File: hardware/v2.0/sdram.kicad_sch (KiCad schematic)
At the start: 10 parts, among them IC1 IS42S16160J-6BLI, U1 ECP5-CABGA256

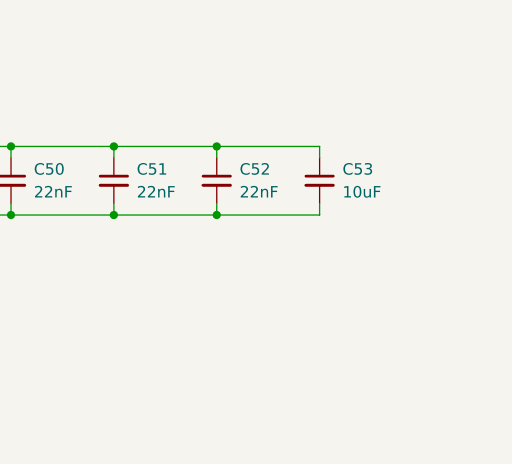
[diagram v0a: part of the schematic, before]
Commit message: Power lines
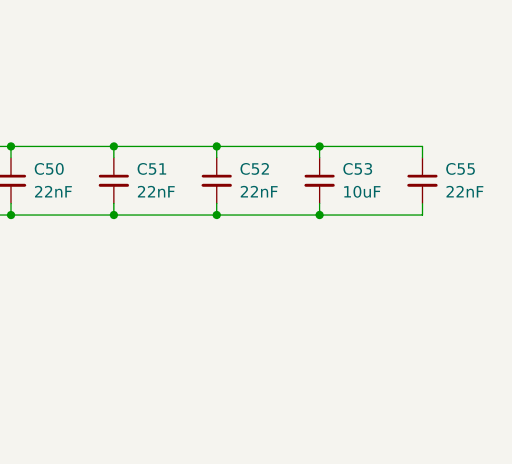
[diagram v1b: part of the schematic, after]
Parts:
- added C55: 22nF, Capacitor_SMD:C_0603_1608Metric, symbol Device:C_Small
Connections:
- net +3V3: now also C55.1
- net GND: now also C55.2
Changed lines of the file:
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@@
 	)
 	(junction
+		(at 264.16 39.37)
+		(diameter 0)
+		(color 0 0 0 0)
+	)
+	(junction
 		(at 53.34 58.42)
 		(diameter 0)
@@
 	)
 	(junction
+		(at 264.16 46.99)
+		(diameter 0)
+		(color 0 0 0 0)
+	)
+	(junction
 		(at 218.44 39.37)
 		(diameter 0)
@@
 	(wire
 		(pts
+			(xy 264.16 39.37) (xy 275.59 39.37)
+		)
+		(stroke
+			(width 0)
+			(type default)
+		)
+	)
+	(wire
+		(pts
 			(xy 54.61 125.73) (xy 60.96 125.73)
 		)
@@
 	(wire
 		(pts
+			(xy 275.59 46.99) (xy 275.59 45.72)
+		)
+		(stroke
+			(width 0)
+			(type default)
+		)
+	)
+	(wire
+		(pts
 			(xy 194.31 39.37) (xy 194.31 40.64)
 		)
@@
 	(wire
 		(pts
+			(xy 275.59 39.37) (xy 275.59 40.64)
+		)
+		(stroke
+			(width 0)
+			(type default)
+		)
+	)
+	(wire
+		(pts
 			(xy 157.48 100.33) (xy 162.56 100.33)
 		)
@@
 		)
 	)
+	(wire
+		(pts
+			(xy 264.16 46.99) (xy 275.59 46.99)
+		)
+		(stroke
+			(width 0)
+			(type default)
+		)
+	)
 	(bus
 		(pts
@@
 				)
 			)
+		)
+	)
+	(symbol
+		(lib_id "Device:C_Small")
+		(at 275.59 43.18 0)
+		(mirror y)
+		(unit 1)
+		(exclude_from_sim no)
+		(in_bom yes)
+		(on_board yes)
+		(dnp no)
+		(fields_autoplaced yes)
+		(property "Reference" "C55"
+			(at 278.13 41.9162 0)
+			(effects
+				(font
+					(size 1.27 1.27)
+				)
+				(justify right)
+			)
+		)
+		(property "Value" "22nF"
+			(at 278.13 44.4562 0)
+			(effects
+				(font
+					(size 1.27 1.27)
+				)
+				(justify right)
+			)
+		)
+		(property "Footprint" "Capacitor_SMD:C_0603_1608Metric"
+			(at 275.59 43.18 0)
+			(effects
+				(font
+					(size 1.27 1.27)
+				)
+				(hide yes)
+			)
+		)
+		(property "Datasheet" "~"
+			(at 275.59 43.18 0)
+			(effects
+				(font
+					(size 1.27 1.27)
+				)
+				(hide yes)
+			)
+		)
+		(property "Description" "Unpolarized capacitor, small symbol"
+			(at 275.59 43.18 0)
+			(effects
+				(font
+					(size 1.27 1.27)
+				)
+				(hide yes)
+			)
+		)
+		(property "LCSC Part #" "C77571"
+			(at 275.59 43.18 0)
+			(effects
+				(font
+					(size 1.27 1.27)
+				)
+				(hide yes)
+			)
+		)
+		(property "LCSC Link" "https://lcsc.com/product-detail/Multilayer-Ceramic-Capacitors-MLCC-SMD-SMT_Samsung-Electro-Mechanics-CL05B104KB54PNC_C307331.html"
+			(at 275.59 43.18 0)
+			(effects
+				(font
+					(size 1.27 1.27)
+				)
+				(hide yes)
+			)
+		)
+		(property "Manufactuer Part Number" "0603B223K500NT"
+			(at 275.59 43.18 0)
+			(effects
+				(font
+					(size 1.27 1.27)
+				)
+				(hide yes)
+			)
+		)
+		(property "Note" ""
+			(at 275.59 43.18 0)
+			(effects
+				(font
+					(size 1.27 1.27)
+				)
+				(hide yes)
+			)
+		)
+		(property "Notes" ""
+			(at 275.59 43.18 0)
+			(effects
+				(font
+					(size 1.27 1.27)
+				)
+				(hide yes)
+			)
+		)
+		(pin "1"
+		)
+		(pin "2"
+		)
+		(instances
+			(project "icepi-zero"
+				(path "/f88da08e-cf42-4d03-a08f-3f602fe6658d/3bffbb9a-e009-498c-a1b0-c490cdf30139"
+					(reference "C55")
+					(unit 1)
+				)
+			)

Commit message: Power lines done
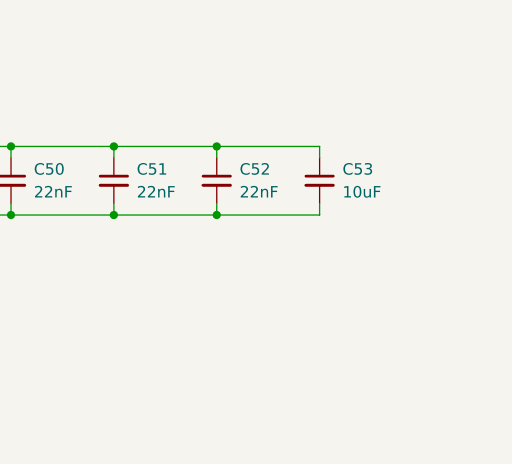
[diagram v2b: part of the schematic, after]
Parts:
- removed C55: 22nF, Capacitor_SMD:C_0603_1608Metric, symbol Device:C_Small
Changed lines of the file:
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@@
 	)
 	(junction
-		(at 264.16 39.37)
-		(diameter 0)
-		(color 0 0 0 0)
-	)
-	(junction
 		(at 53.34 58.42)
 		(diameter 0)
@@
 	)
 	(junction
-		(at 264.16 46.99)
-		(diameter 0)
-		(color 0 0 0 0)
-	)
-	(junction
 		(at 218.44 39.37)
 		(diameter 0)
@@
 	(wire
 		(pts
-			(xy 264.16 39.37) (xy 275.59 39.37)
-		)
-		(stroke
-			(width 0)
-			(type default)
-		)
-	)
-	(wire
-		(pts
 			(xy 54.61 125.73) (xy 60.96 125.73)
 		)
@@
 	(wire
 		(pts
-			(xy 275.59 46.99) (xy 275.59 45.72)
-		)
-		(stroke
-			(width 0)
-			(type default)
-		)
-	)
-	(wire
-		(pts
 			(xy 194.31 39.37) (xy 194.31 40.64)
 		)
@@
 	(wire
 		(pts
-			(xy 275.59 39.37) (xy 275.59 40.64)
-		)
-		(stroke
-			(width 0)
-			(type default)
-		)
-	)
-	(wire
-		(pts
 			(xy 157.48 100.33) (xy 162.56 100.33)
 		)
@@
 		)
 	)
-	(wire
-		(pts
-			(xy 264.16 46.99) (xy 275.59 46.99)
-		)
-		(stroke
-			(width 0)
-			(type default)
-		)
-	)
 	(bus
 		(pts
@@
 				)
 			)
-		)
-	)
-	(symbol
-		(lib_id "Device:C_Small")
-		(at 275.59 43.18 0)
-		(mirror y)
-		(unit 1)
-		(exclude_from_sim no)
-		(in_bom yes)
-		(on_board yes)
-		(dnp no)
-		(fields_autoplaced yes)
-		(property "Reference" "C55"
-			(at 278.13 41.9162 0)
-			(effects
-				(font
-					(size 1.27 1.27)
-				)
-				(justify right)
-			)
-		)
-		(property "Value" "22nF"
-			(at 278.13 44.4562 0)
-			(effects
-				(font
-					(size 1.27 1.27)
-				)
-				(justify right)
-			)
-		)
-		(property "Footprint" "Capacitor_SMD:C_0603_1608Metric"
-			(at 275.59 43.18 0)
-			(effects
-				(font
-					(size 1.27 1.27)
-				)
-				(hide yes)
-			)
-		)
-		(property "Datasheet" "~"
-			(at 275.59 43.18 0)
-			(effects
-				(font
-					(size 1.27 1.27)
-				)
-				(hide yes)
-			)
-		)
-		(property "Description" "Unpolarized capacitor, small symbol"
-			(at 275.59 43.18 0)
-			(effects
-				(font
-					(size 1.27 1.27)
-				)
-				(hide yes)
-			)
-		)
-		(property "LCSC Part #" "C77571"
-			(at 275.59 43.18 0)
-			(effects
-				(font
-					(size 1.27 1.27)
-				)
-				(hide yes)
-			)
-		)
-		(property "LCSC Link" "https://lcsc.com/product-detail/Multilayer-Ceramic-Capacitors-MLCC-SMD-SMT_Samsung-Electro-Mechanics-CL05B104KB54PNC_C307331.html"
-			(at 275.59 43.18 0)
-			(effects
-				(font
-					(size 1.27 1.27)
-				)
-				(hide yes)
-			)
-		)
-		(property "Manufactuer Part Number" "0603B223K500NT"
-			(at 275.59 43.18 0)
-			(effects
-				(font
-					(size 1.27 1.27)
-				)
-				(hide yes)
-			)
-		)
-		(property "Note" ""
-			(at 275.59 43.18 0)
-			(effects
-				(font
-					(size 1.27 1.27)
-				)
-				(hide yes)
-			)
-		)
-		(property "Notes" ""
-			(at 275.59 43.18 0)
-			(effects
-				(font
-					(size 1.27 1.27)
-				)
-				(hide yes)
-			)
-		)
-		(pin "1"
-		)
-		(pin "2"
-		)
-		(instances
-			(project "icepi-zero"
-				(path "/f88da08e-cf42-4d03-a08f-3f602fe6658d/3bffbb9a-e009-498c-a1b0-c490cdf30139"
-					(reference "C55")
-					(unit 1)
-				)
-			)
